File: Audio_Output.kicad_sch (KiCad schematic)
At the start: 8 parts, among them J9 Conn_02x04_Odd_Even, U8 MAX98357AGTE_V+T

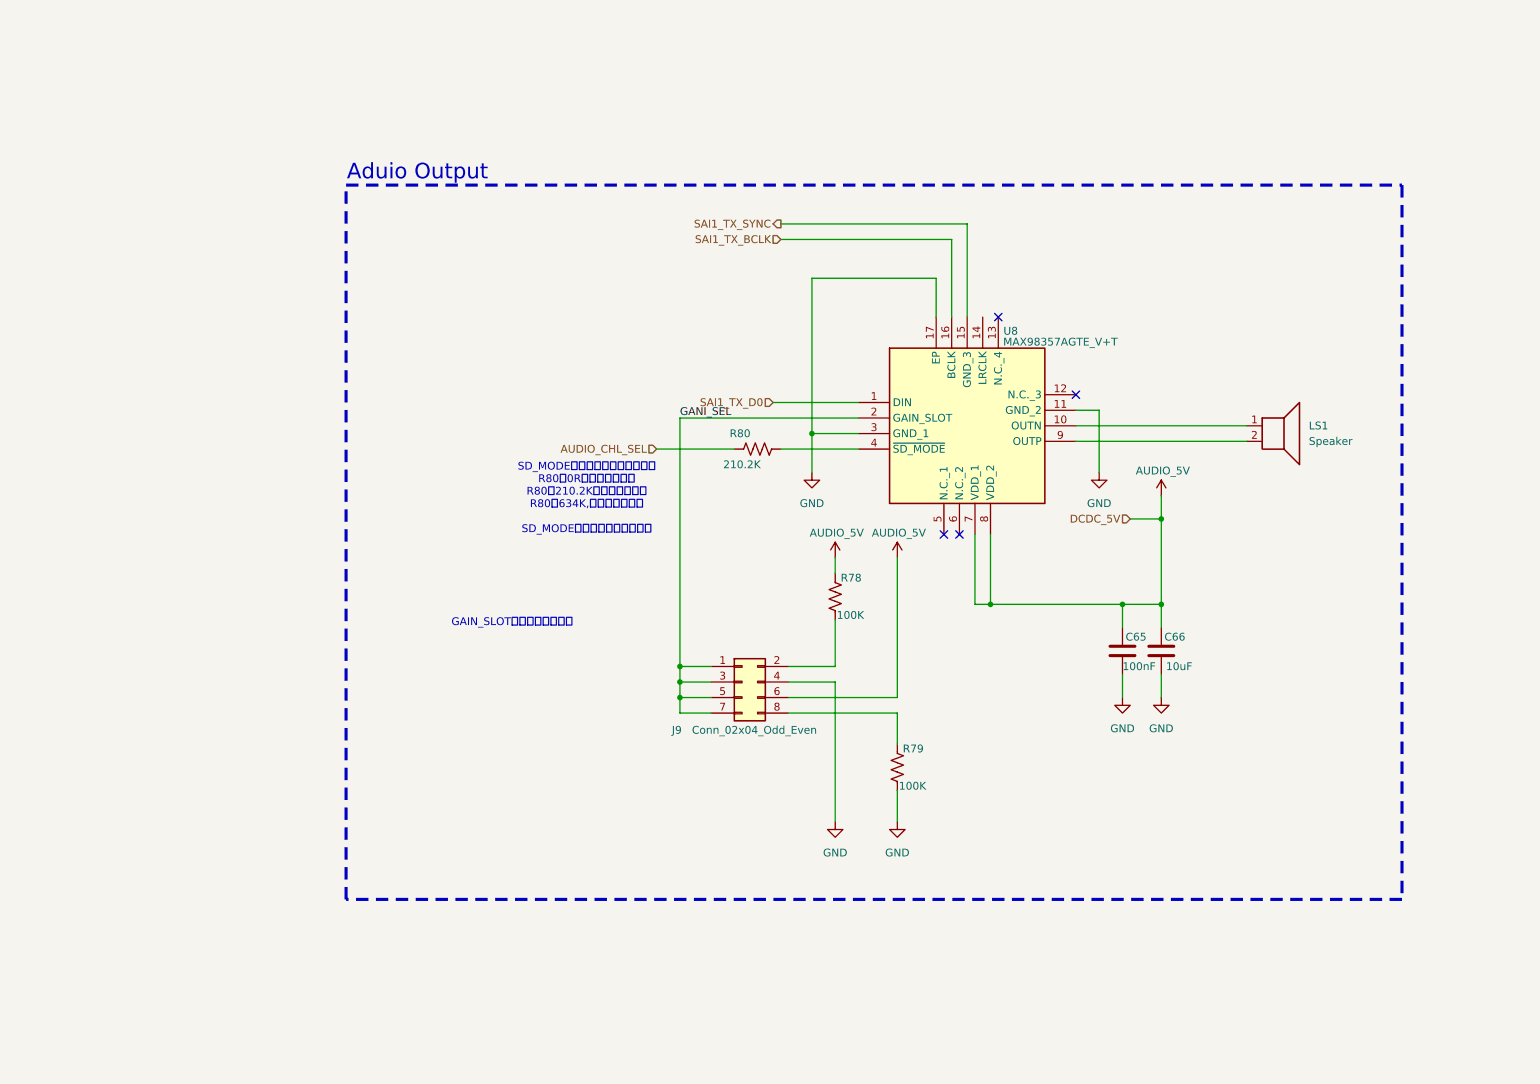
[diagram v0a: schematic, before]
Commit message: 2026 08 24 画图完成，准备生产
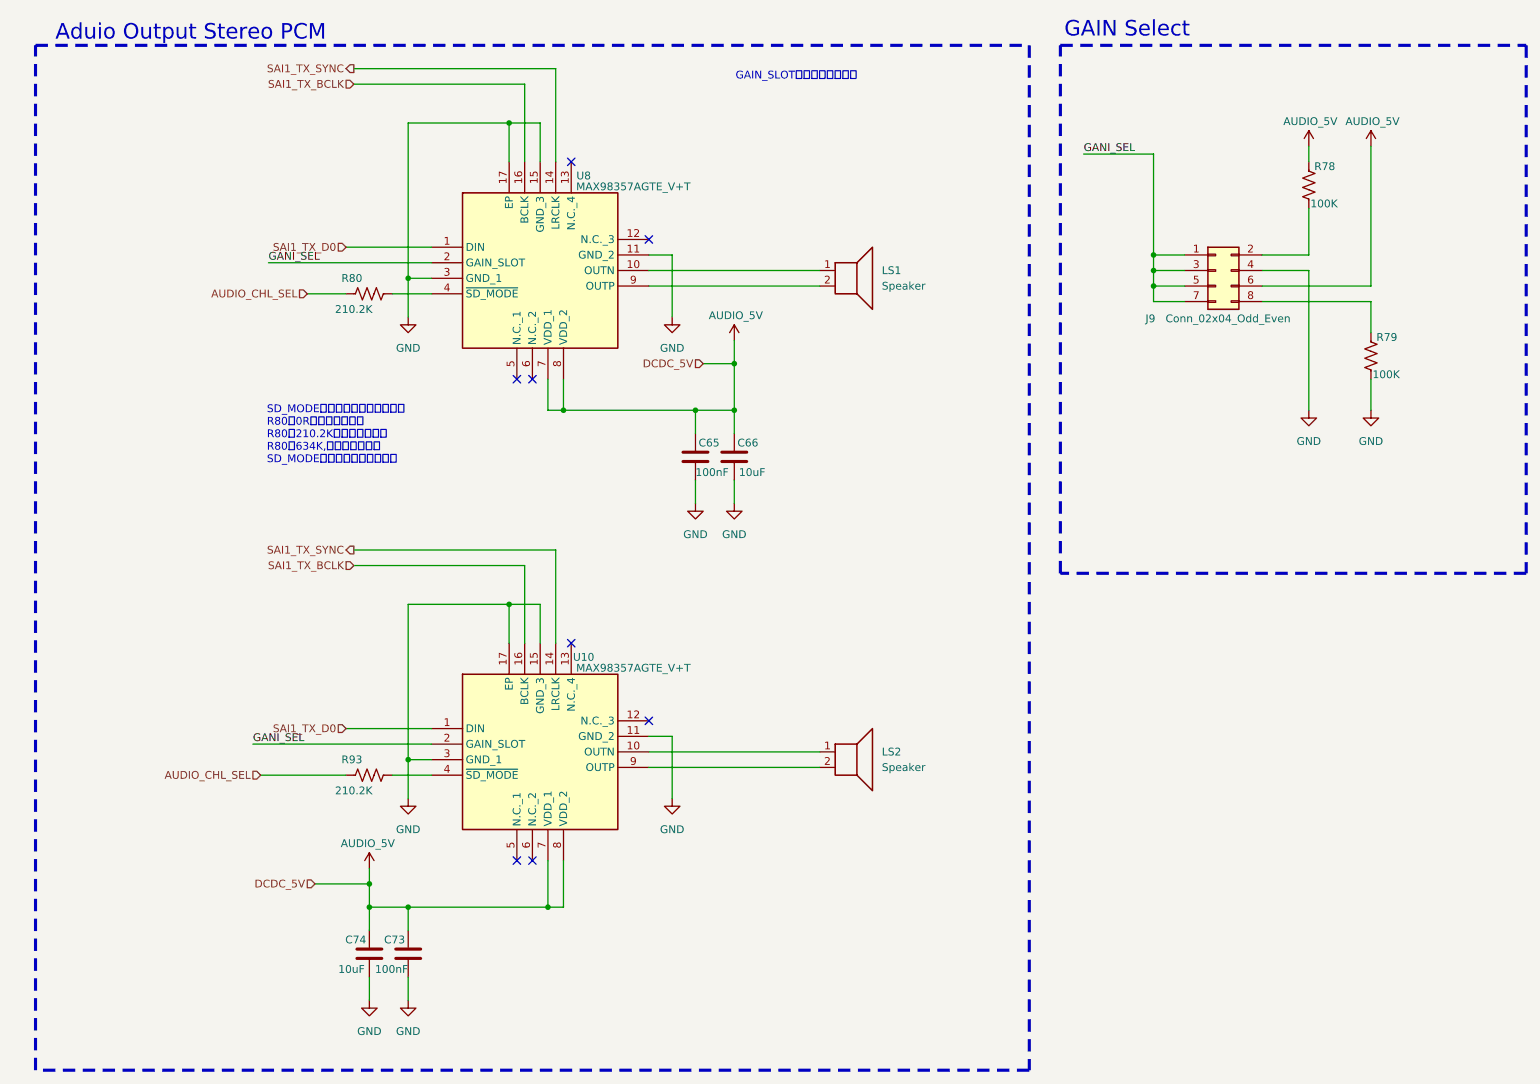
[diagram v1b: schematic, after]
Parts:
- added C73: 100nF, Capacitor_SMD:C_0603_1608Metric_Pad1.08x0.95mm_HandSolder, symbol Device:C
- added C74: 10uF, Capacitor_SMD:C_0805_2012Metric_Pad1.18x1.45mm_HandSolder, symbol Device:C
- added LS2: Speaker, Connector_JST:JST_PH_S2B-PH-K_1x02_P2.00mm_Horizontal, symbol Device:Speaker
- added R93: 210.2K, Resistor_SMD:R_0603_1608Metric_Pad0.98x0.95mm_HandSolder, symbol Device:R_US
- added U10: MAX98357AGTE_V+T, Package_DFN_QFN:TQFN-16-1EP_3x3mm_P0.5mm_EP1.23x1.23mm_ThermalVias, symbol UPT:MAX98357AGTE_V+T
- C65: footprint Capacitor_SMD:C_0805_2012Metric_Pad1.18x1.45mm_HandSolder -> Capacitor_SMD:C_0603_1608Metric_Pad1.08x0.95mm_HandSolder
- LS1: footprint Resistor_SMD:R_2816_7142Metric_Pad3.20x4.45mm_HandSolder -> Connector_JST:JST_PH_S2B-PH-K_1x02_P2.00mm_Horizontal
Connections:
- net AUDIO_5V: now also C73.1, C74.1, U10.7 (VDD_1), U10.8 (VDD_2)
- net AUDIO_CHL_SEL: now also R93.2
- net GANI_SEL: now also U10.2 (GAIN_SLOT)
- net GND: now also U8.15 (GND_3), C73.2, C74.2, U10.11 (GND_2), U10.15 (GND_3), U10.17 (EP), U10.3 (GND_1)
- net SAI1_TX_BCLK: now also U10.16 (BCLK)
- net SAI1_TX_D0: now also U10.1 (DIN)
- net SAI1_TX_SYNC: now also U8.14 (LRCLK), U10.14 (LRCLK); no longer U8.15 (GND_3)
- new net: LS2.1, U10.10 (OUTN)
- new net: R93.1, U10.4 (~{SD_MODE})
- new net: LS2.2, U10.9 (OUTP)
- no-connect marks 4 -> 8
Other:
- note added: "Aduio Output Stereo PCM"
- note added: "GAIN Select"
- note removed: "Aduio Output"
- moved on the sheet: C65, C66, LS1, R80, U8
